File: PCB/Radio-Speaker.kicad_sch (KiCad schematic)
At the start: 9 parts, among them CN1 PJ-3200, U1 RDA5807MRRD-102V2.0, U2 XIAO-RP2040-DIP, U3 TDA2822NBD

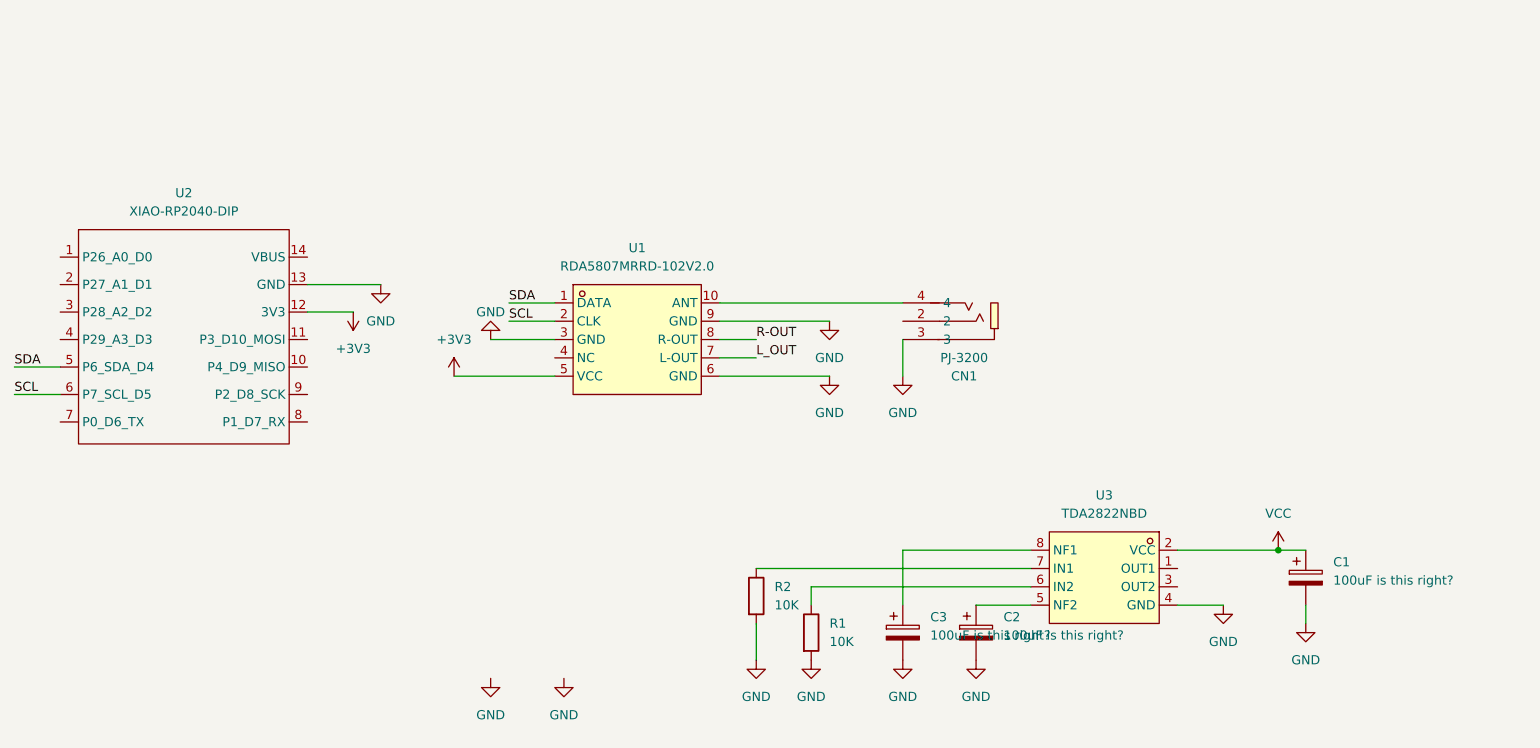
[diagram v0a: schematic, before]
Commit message: PCB work
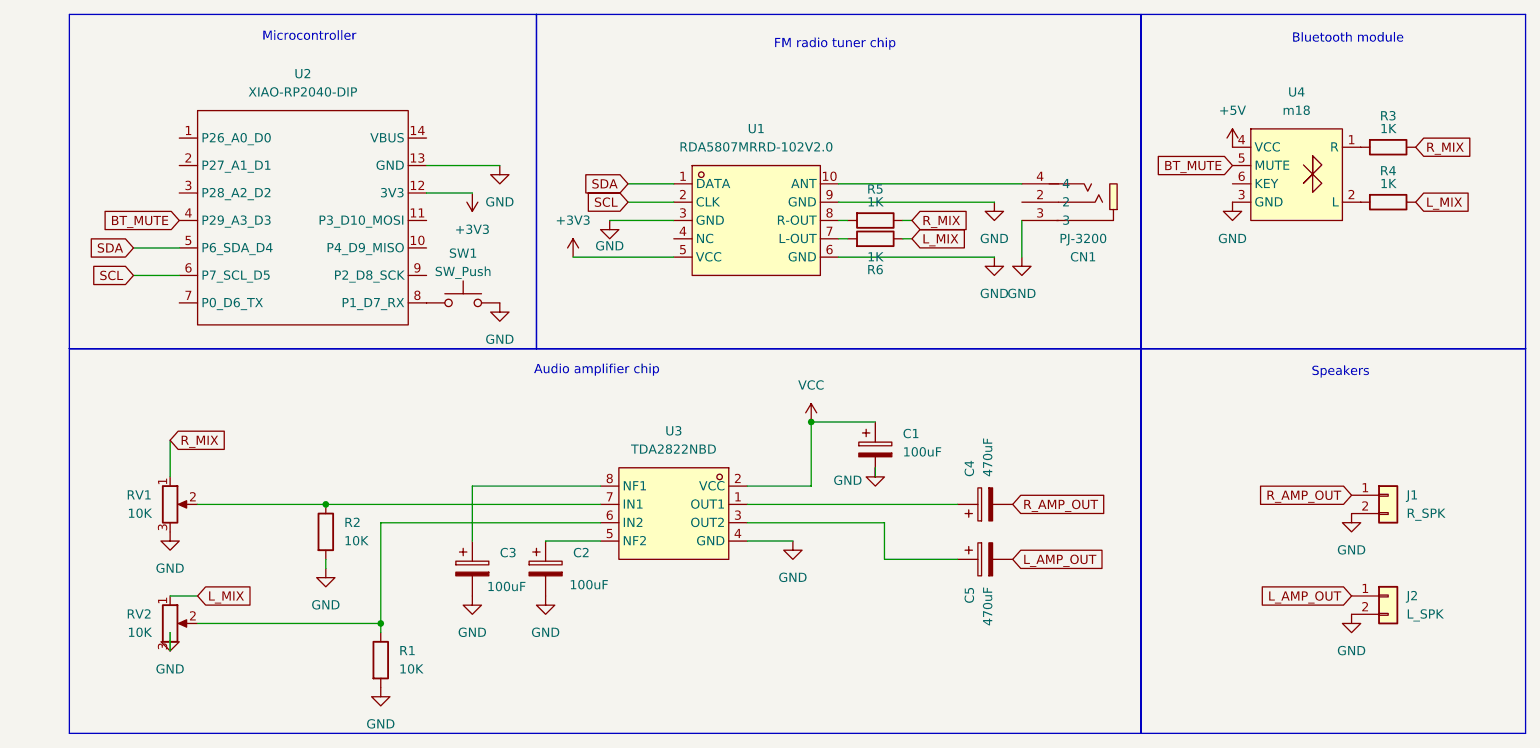
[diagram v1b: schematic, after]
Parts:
- added C4, C5: 470uF, Capacitor_THT:CP_Radial_D6.3mm_P2.50mm, symbol Device:C_Polarized
- added J1: R_SPK, Connector_PinHeader_2.54mm:PinHeader_1x02_P2.54mm_Vertical, symbol Connector_Generic:Conn_01x02
- added J2: L_SPK, Connector_PinHeader_2.54mm:PinHeader_1x02_P2.54mm_Vertical, symbol Connector_Generic:Conn_01x02
- added R3, R4, R5, R6: 1K, Resistor_THT:R_Axial_DIN0207_L6.3mm_D2.5mm_P7.62mm_Horizontal, symbol Device:R
- added RV1, RV2: 10K, Connector_PinHeader_2.54mm:PinHeader_1x03_P2.54mm_Vertical, symbol Device:R_Potentiometer
- added SW1: SW_Push, Connector_PinHeader_2.54mm:PinHeader_1x02_P2.54mm_Vertical, symbol Switch:SW_Push
- added U4: m18, Static:m18, symbol m18:m18
- C1, C2, C3: value 100uF is this right? -> 100uF; footprint (none) -> Capacitor_THT:CP_Radial_D6.3mm_P2.50mm
- CN1: footprint easyeda2kicad:AUDIO-TH_PJ-3200 -> Static:AUDIO-TH_PJ-3200
- R1, R2: footprint (none) -> Resistor_THT:R_Axial_DIN0207_L6.3mm_D2.5mm_P7.62mm_Horizontal
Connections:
- net GND: now also J1.2 (Pin_2), J2.2 (Pin_2), RV1.3, RV2.3, SW1.2, U4.3 (GND)
- net at R1.1, U3.6 (IN2): now also RV2.2
- net at U3.1 (OUT1): now also C4.1
- net at U3.3 (OUT2): now also C5.1
- net at R2.1, U3.7 (IN1): now also RV1.2
- net BT_MUTE: now reaches U2.4 (P29_A3_D3)
- net BT_MUTE: now also U4.5 (MUTE)
- net at U2.8 (P1_D7_RX): now also SW1.1
- net L_OUT: no longer names the net of U1.7 (L-OUT)
- net L_OUT: now also R6.2
- net R-OUT: no longer names the net of U1.8 (R-OUT)
- net R-OUT: now also R5.2
- new net: R3.2, U4.1 (R)
- new net: R4.2, U4.2 (L)
- new net +5V: U4.4 (VCC)
- new net L_AMP_OUT: C5.2, J2.1 (Pin_1)
- new net L_MIX: R4.1, R6.1, RV2.1
- new net R_AMP_OUT: C4.2, J1.1 (Pin_1)
- new net R_MIX: R3.1, R5.1, RV1.1
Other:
- note added: "Audio amplifier chip"
- note added: "Bluetooth module"
- note added: "FM radio tuner chip"
- note added: "Microcontroller"
- note added: "Speakers"
- moved on the sheet: C1, C2, C3, CN1, R1, R2, U1, U2, U3
